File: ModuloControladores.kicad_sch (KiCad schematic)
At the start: 24 parts, among them J13 Borner ESP32, J14 Conn. Conv. HV, J15 Conn. Conv. LV, J16 Conn. ESP32, J17 Conn. LED Tr., J18 Conn. LED Empot., J19 Conn. LED Polea, J20 Conn. LED Lineal, J21 Conn. Ctrl. Tr., J22 Conn. Ctrl. Polea, J23 Conn. Ctrl. Empot. 2, J24 Conn. Ctrl. Empot. 1, J25 Borner Drivers

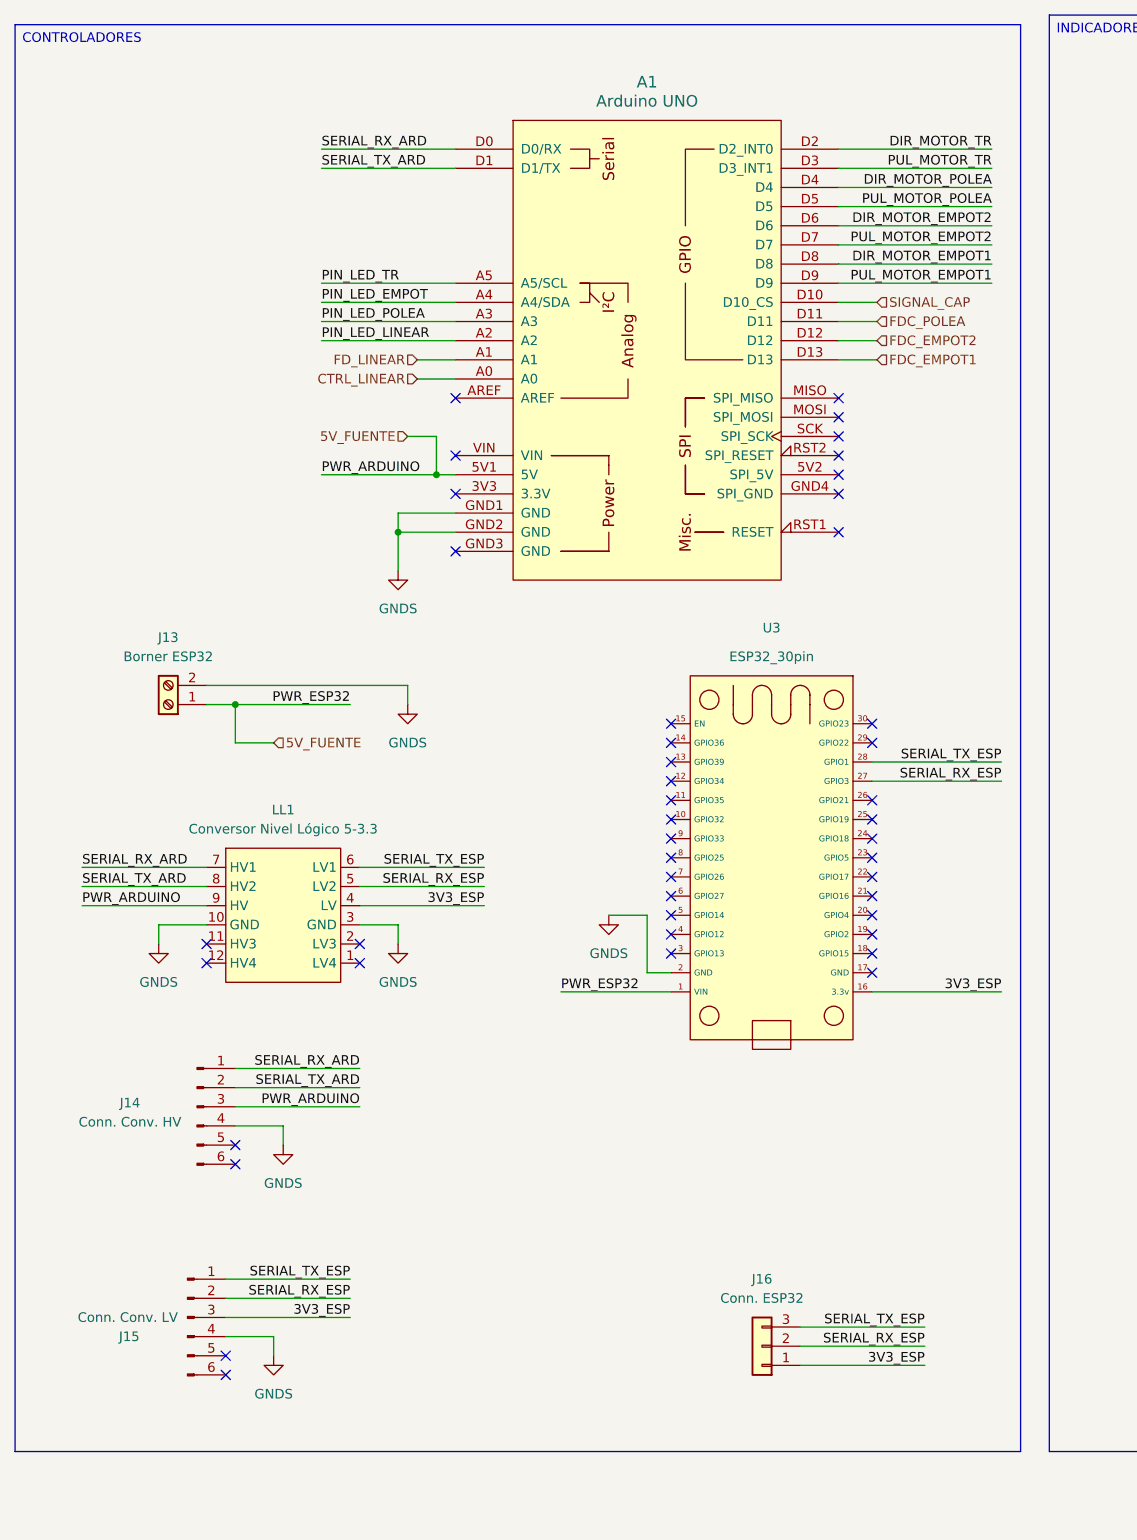
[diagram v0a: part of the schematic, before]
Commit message: Nuevo step y pdf
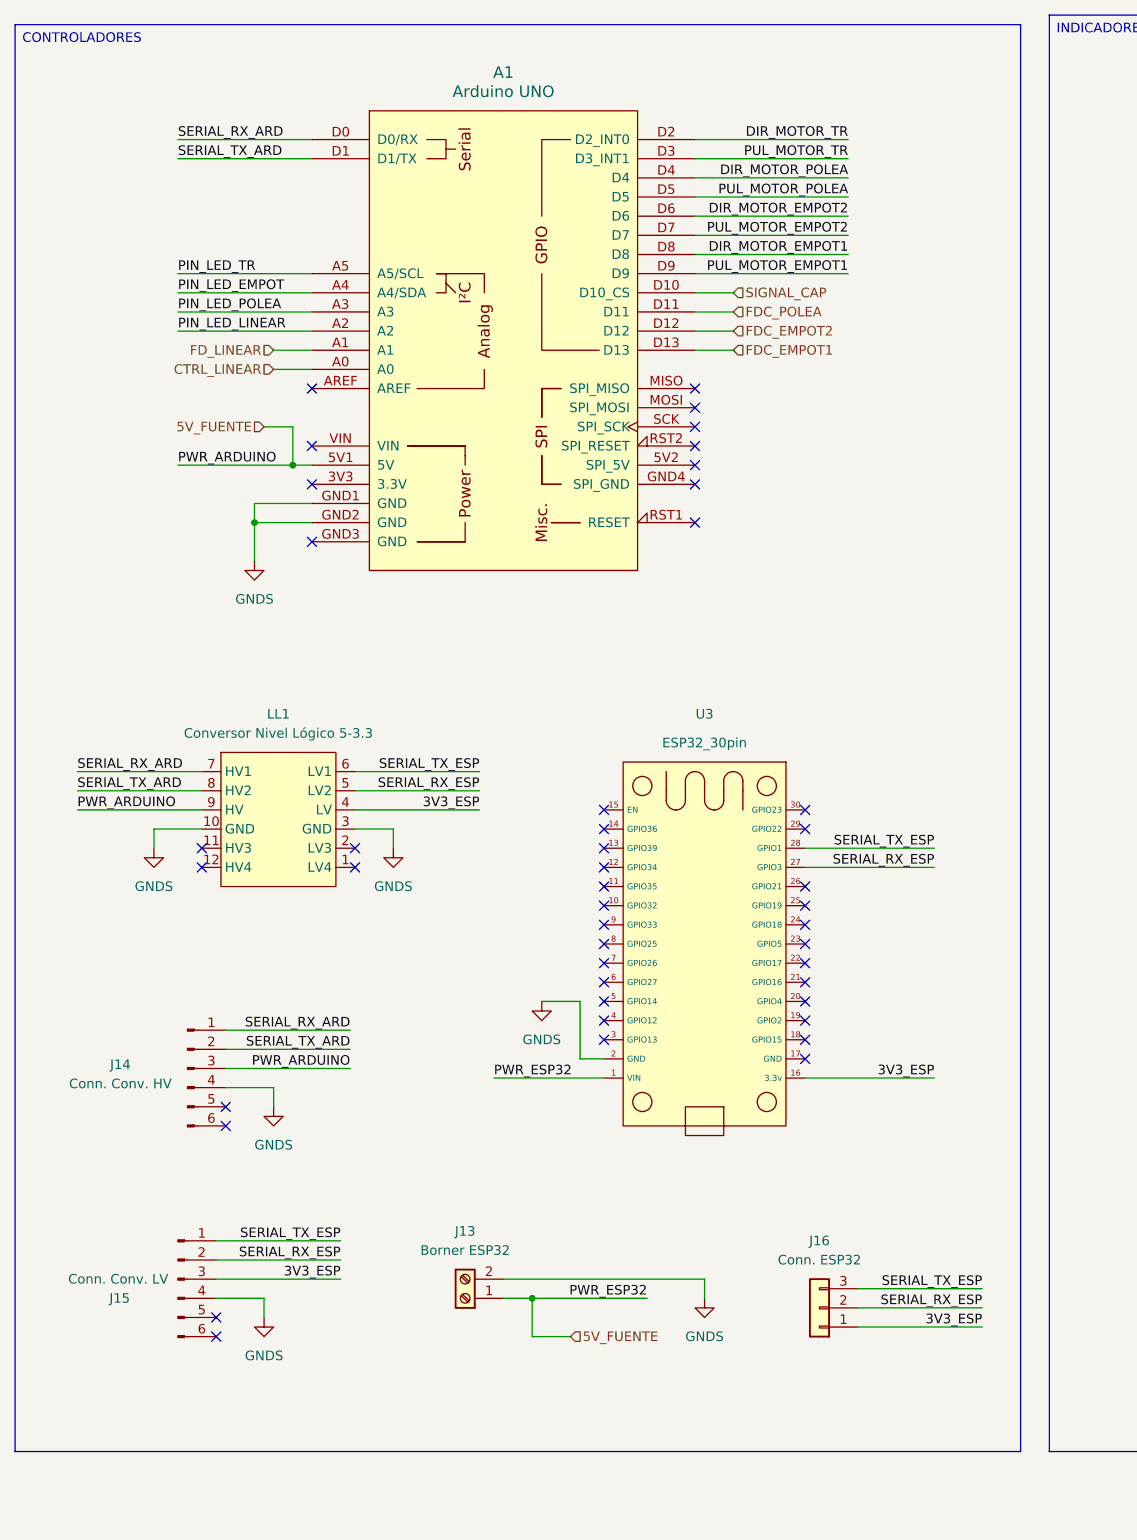
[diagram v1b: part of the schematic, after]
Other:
- moved on the sheet: A1, J13, J14, J15, J16, LL1, U3
